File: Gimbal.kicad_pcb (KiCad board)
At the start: 2 copper layers, 76.2 x 63.5 mm, 41 parts, among them J1 Conn_01x03, J2 USB_C_Receptacle_USB2.0, J3 0022232041, J4 0022232041, J5 0022232041, J6 Conn_01x02, Q1 Q_NPN_BCE, Q2 Q_NPN_BCE, SW1 SW_Push, U1 ESP32-S2-SOLO, U2 BMI088, U3 CP2102N-Axx-xQFN28, U4 TLV70433DBVT, U5 DRV8846RGET, U6 DRV8846RGET

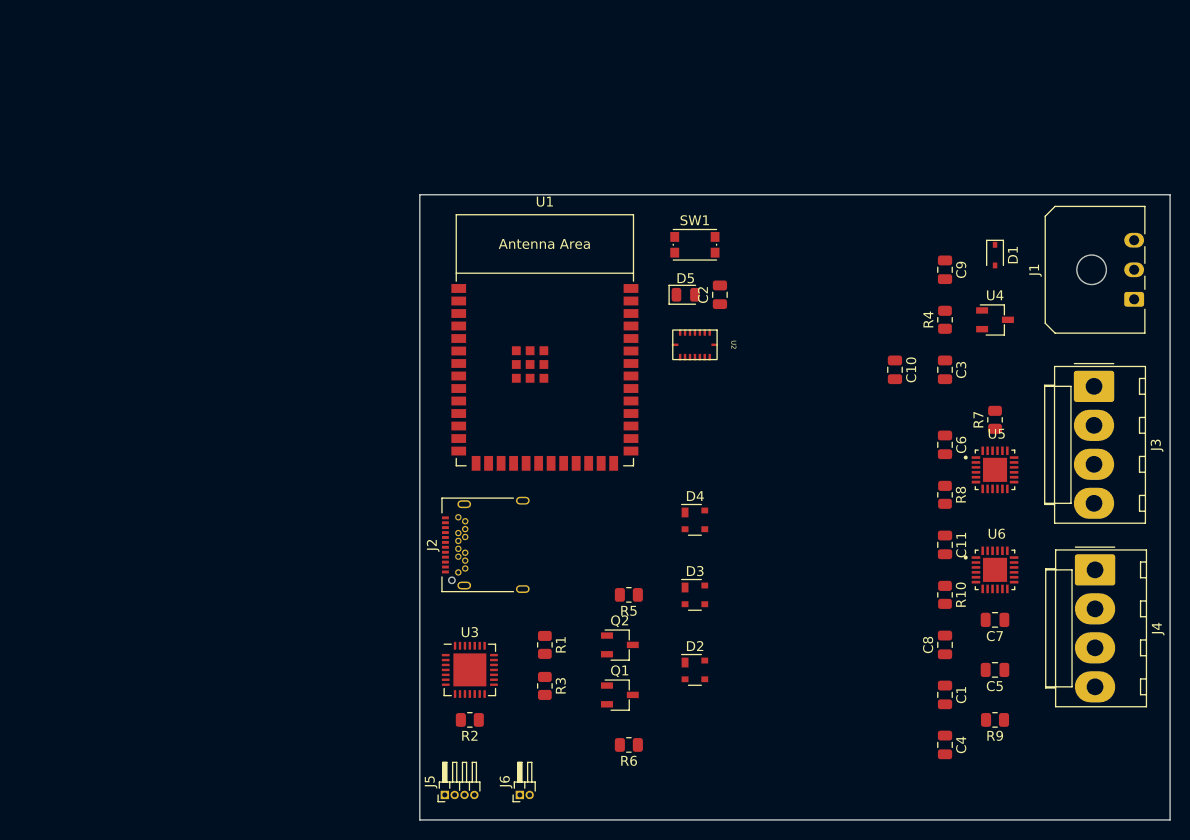
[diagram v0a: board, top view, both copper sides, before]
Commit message: prelim routing
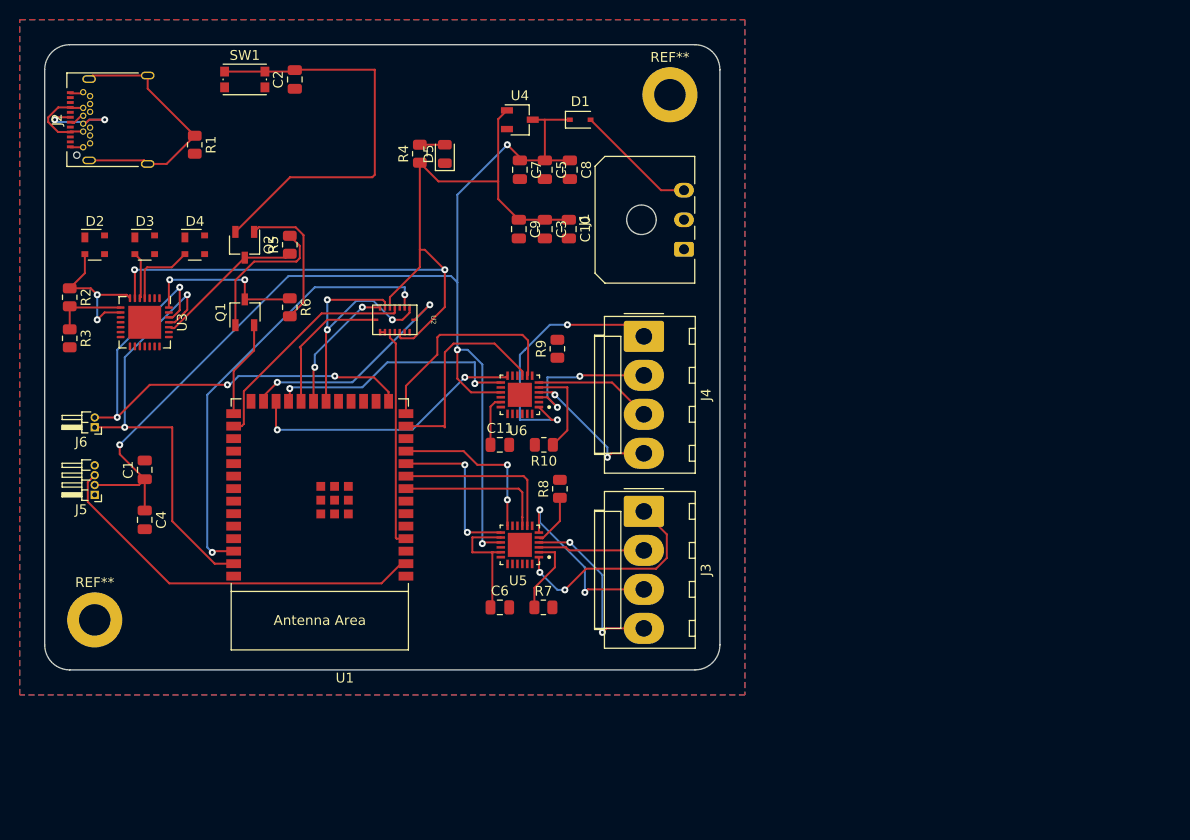
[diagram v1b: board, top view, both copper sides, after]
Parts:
- added REF**: MountingHole_3.2mm_M3_DIN965_Pad, MountingHole:MountingHole_3.2mm_M3_DIN965_Pad, F.Cu at (177.8, 66.0)
- added REF**: MountingHole_3.2mm_M3_DIN965_Pad, MountingHole:MountingHole_3.2mm_M3_DIN965_Pad, F.Cu at (119.4, 119.4)
- moved C1 84.4 mm to (124.5, 104.1), turned to 90 degrees
- moved C4 84.4 mm to (124.5, 109.2)
- moved D2 74.7 mm to (119.4, 81.3)
- moved C5 68.3 mm to (165.1, 73.7), turned to -90 degrees
- moved C7 66.5 mm to (162.6, 73.7), turned to -90 degrees
- moved D3 66.2 mm to (124.5, 81.3)
- moved R1 62.0 mm to (129.5, 71.1)
- moved C8 61.5 mm to (167.6, 73.7), turned to -90 degrees
- moved R3 59.8 mm to (116.8, 90.8)
- moved R2 59.1 mm to (116.8, 86.6), turned to -90 degrees
- moved R9 58.3 mm to (166.4, 91.8), turned to 90 degrees
- moved D4 58.0 mm to (129.5, 81.3)
- moved J2 57.6 mm to (121.9, 68.6)
- moved J6 57.1 mm to (119.4, 99.8), turned to 180 degrees
- moved R6 56.2 mm to (139.2, 87.6), turned to -90 degrees
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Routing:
- net +3V3: track 0.00 -> 129.7 mm, vias 0 -> 2
- net +12V: track 0.00 -> 123.9 mm, vias 0 -> 4
- net /ESPRX: track 0.00 -> 52.9 mm, vias 0 -> 4
- net /ESPTX: track 0.00 -> 45.4 mm, vias 0 -> 2
- net /ESPIO2: track 0.00 -> 45.1 mm, vias 0 -> 2
- net /EN: track 0.00 -> 42.6 mm
- net /Motor2Step: track 0.00 -> 28.6 mm, vias 0 -> 2
- net /SPI_MISO: track 0.00 -> 28.1 mm, vias 0 -> 3
- net /Motor2Out1: track 0.00 -> 27.2 mm, vias 0 -> 2
- net Net-(J2-PadS1): track 0.00 -> 26.3 mm
- net /Motor2Dir: track 0.00 -> 26.1 mm, vias 0 -> 2
- net /VBUS: track 0.00 -> 24.3 mm, vias 0 -> 2
- net /ESPIO35: track 0.00 -> 23.6 mm
- net /ESPIO34: track 0.00 -> 23.4 mm, vias 0 -> 2
- net /Motor2M0: track 0.00 -> 22.3 mm
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- added copper zone on B.Cu, net GND
- added copper zone on F.Cu, net GND
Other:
- board size 76.2 x 63.5 mm -> 68.6 x 63.5 mm
